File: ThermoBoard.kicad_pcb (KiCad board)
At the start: 4 copper layers, 72.5 x 69 mm, 181 parts, among them J100 Conn_01x05_Pin, J101 Conn_01x03, J102 Conn_01x03, J103 Screw_Terminal_01x02, J104 USB_C_Receptacle_USB2.0_16P, J105 PCC-SMP-K-5, J106 PCC-SMP-K-5, J107 PCC-SMP-K-5, J108 PCC-SMP-K-5, J200 RJ45_Hanrun_HR911105A_Horizon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, SW100 SW_Push, U100 STM32H563RITx, U101 AP2112K-3.3, U102 USBLC6-2SC6, U200 LAN8742A, U201 USBLC6-4SC6, U300 MAX31856, U301 MAX31856, U302 MAX31856, U303 MAX31856, U400 TJA1042T-3, Y100 X322516MMB4SI, Y200 25MHz

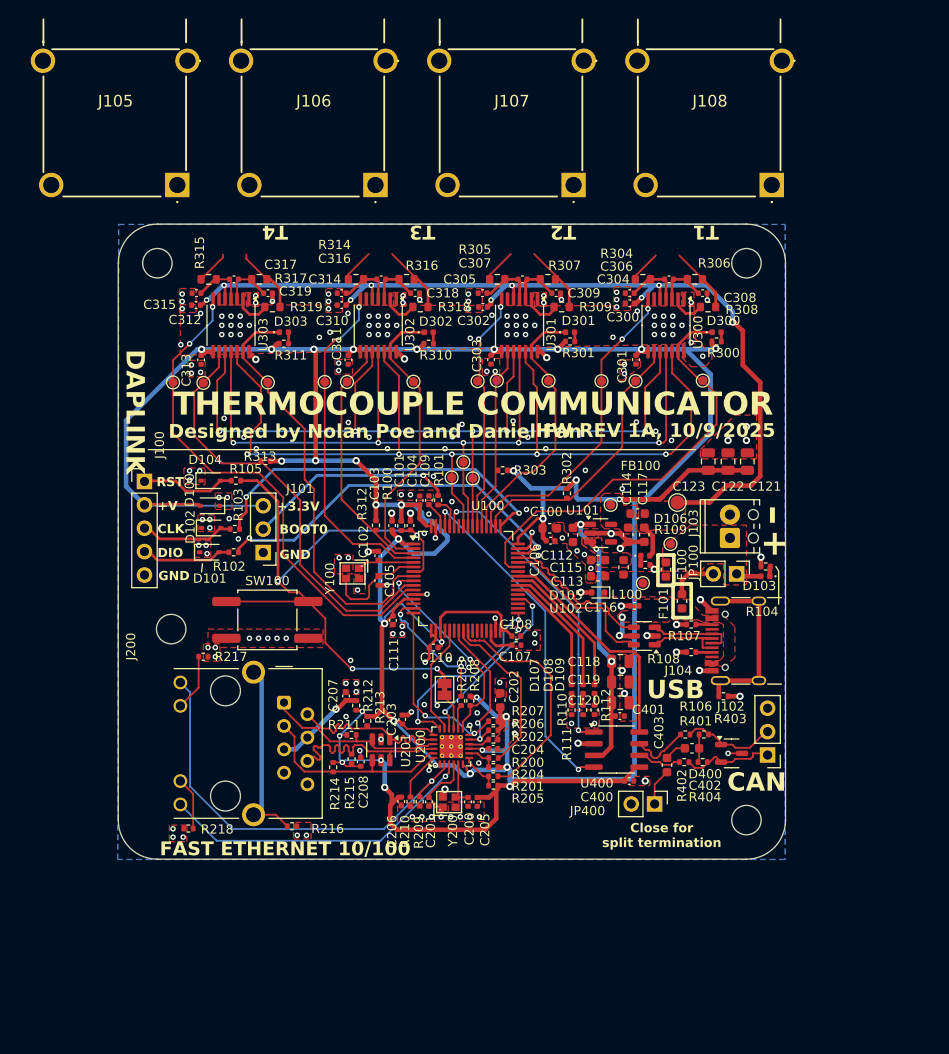
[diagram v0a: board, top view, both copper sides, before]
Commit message: First workable layout
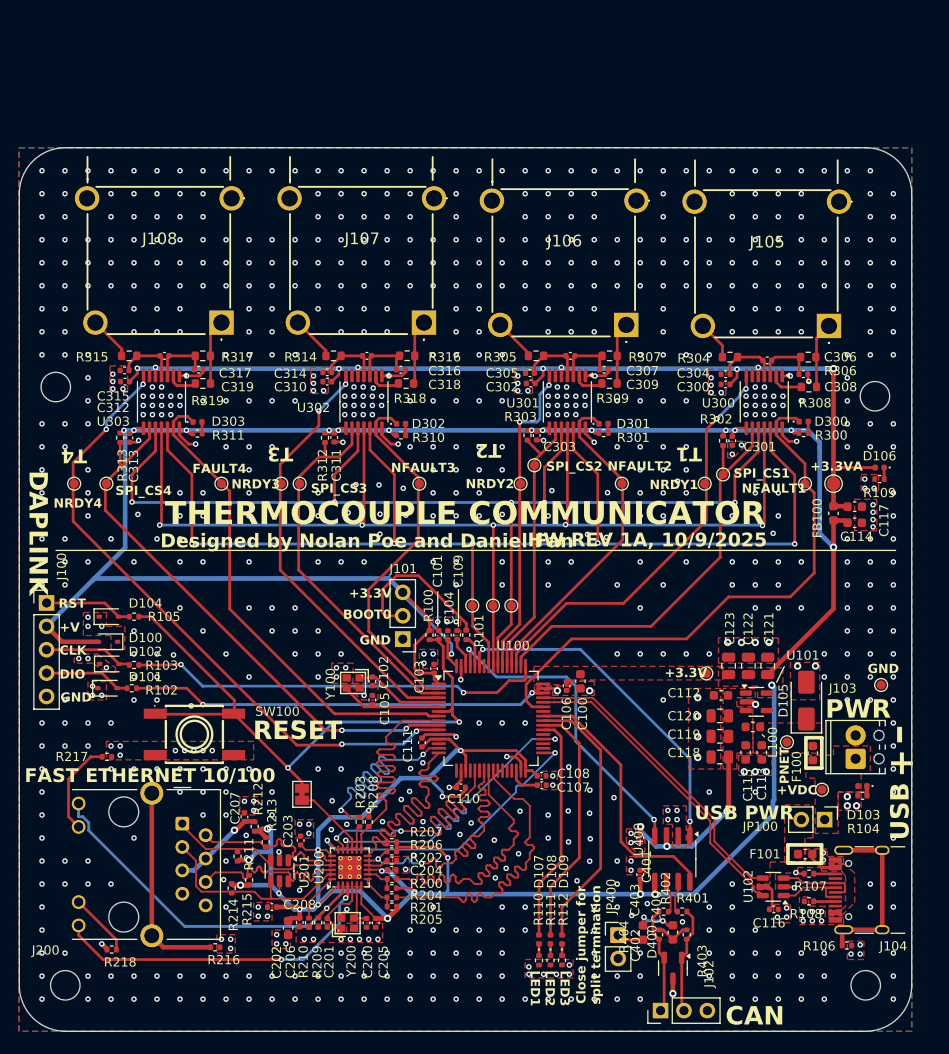
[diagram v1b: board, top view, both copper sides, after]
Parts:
- added TP112: TestPoint_Small, TestPoint:TestPoint_Pad_D1.0mm, F.Cu at (184.1, 115.1)
- C200, C201: value 5p6 -> 10p
- D105: value 1N4148WT -> MRA4007T3G; footprint Diode_SMD:D_SOD-523 -> Diode_SMD:D_SMA
- SW100: value SW_Push -> K2-1157SP-I4SW-04; footprint Button_Switch_SMD:SW_Push_1P1T_NO_CK_KSC6xxG -> Library:SW-SMD_4P-L6.2-W6.2-P4.50-LS8.6
- moved J105 72.4 mm to (178.5, 76.1)
- moved J108 61.6 mm to (112.5, 75.7)
- moved H4 40.4 mm to (95.5, 147.7)
- moved C116 36.3 mm to (172.5, 139.4), turned to 180 degrees
- moved C202 33.8 mm to (119.7, 141.5), turned to -90 degrees
- moved TP101 31.4 mm to (177.7, 126.5)
- moved J106 31.2 mm to (156.4, 76.0)
- moved U102 30.6 mm to (172.4, 137.0)
- moved F101 30.6 mm to (175.9, 133.4), turned to 0 degrees
- moved R106 30.2 mm to (180.4, 143.4)
- moved J104 30.2 mm to (183.2, 137.3)
- moved J102 30.1 mm to (160.2, 150.4), turned to 90 degrees
- moved R107 29.9 mm to (176.3, 135.6)
- moved R108 29.9 mm to (176.3, 138.6)
- moved JP100 28.4 mm to (178.0, 129.7)
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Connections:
- net Net-(JP100-B) renamed /Microcontroller/USB_FUSE
- J107 pad 1: /Thermocouples/T1_IN- -> /Thermocouples/T3_IN-
- J107 pad 2: /Thermocouples/T1_IN+ -> /Thermocouples/T3_IN+
- SW100 pad 1: GND -> NRST
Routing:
- net SPI_MOSI: track 103.6 -> 134.1 mm
- net SPI_MISO: track 95.8 -> 122.4 mm
- net SPI_SCK: track 93.4 -> 120.0 mm
- net +3V3: track 426.5 -> 405.7 mm, vias 34 -> 31
- net ETH_TX_EN: track 12.1 -> 32.9 mm, vias 0 -> 2
- net ETH_CRS_DV: track 16.4 -> 34.1 mm
- net ETH_RXD0: track 18.6 -> 36.0 mm
- net /Microcontroller/USB_D-: track 17.6 -> 34.2 mm
- net ETH_TXD1: track 19.3 -> 35.8 mm
- net ETH_REF_CLK: track 14.6 -> 30.7 mm
- net /Microcontroller/USB_D+: track 17.6 -> 33.4 mm
- net SPI_CS1: track 29.8 -> 45.2 mm
- net ETH_MDIO: track 20.6 -> 36.0 mm, vias 2 -> 0
- net NFAULT1: track 46.9 -> 61.2 mm
- net SPI_CS3: track 27.4 -> 41.5 mm
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- added copper zone on F.Cu, net /Microcontroller/USB_FUSE
- removed copper zone on F.Cu, net +3.3VA
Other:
- board size 72.5 x 69 mm -> 97 x 96 mm
- board text added: "+3.3VA"
- board text added: "+VDC"
- board text added: "Close jumper for split termination"
- board text added: "FAULT4"
- board text added: "LED3 LED2 LED1"
- board text added: "NFAULT1"
- board text added: "NFAULT2"
- board text added: "NFAULT3"
- board text added: "NRDY1"
- board text added: "NRDY2"
- board text added: "NRDY3"
- board text added: "NRDY4"
- board text added: "PNET"
- board text added: "PWR"
- board text added: "RESET"
- board text added: "SPI_CS1"
- board text added: "SPI_CS2"
- board text added: "SPI_CS3"
- board text added: "SPI_CS4"
- board text added: "USB PWR"
- board text added: "{ "ViaStitching": "0.2", "stitch_zone_0": { "HSpacing": "2.5", "VSpacing": "2.5", "HOffset": "0", "VOffset": "0", "Clearance": ".5", "Randomize": false } }"
- board text removed: "Close for split termination"
